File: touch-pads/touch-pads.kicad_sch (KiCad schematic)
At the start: 47 parts, among them J1 Conn_01x06_Pin, J2 Conn_01x06_Socket, J3 Conn_01x06_Pin, K1 Conn_01x01, K10 Conn_01x01, K11 Conn_01x01, K12 Conn_01x01, K13 Conn_01x01, K14 Conn_01x01, K15 Conn_01x01, K16 Conn_01x01, K17 Conn_01x01, K18 Conn_01x01, K19 Conn_01x01, K2 Conn_01x01, K20 Conn_01x01, K21 Conn_01x01, K22 Conn_01x01, K23 Conn_01x01, K24 Conn_01x01, K25 Conn_01x01, K26 Conn_01x01, K27 Conn_01x01, K28 Conn_01x01, K29 Conn_01x01, K3 Conn_01x01, K30 Conn_01x01, K31 Conn_01x01, K32 Conn_01x01, K4 Conn_01x01, K5 Conn_01x01, K6 Conn_01x01, K7 Conn_01x01, K8 Conn_01x01, K9 Conn_01x01, U10 CAP1188-1-CP-TR, U11 CAP1188-1-CP-TR, U8 CAP1188-1-CP-TR, U9 CAP1188-1-CP-TR

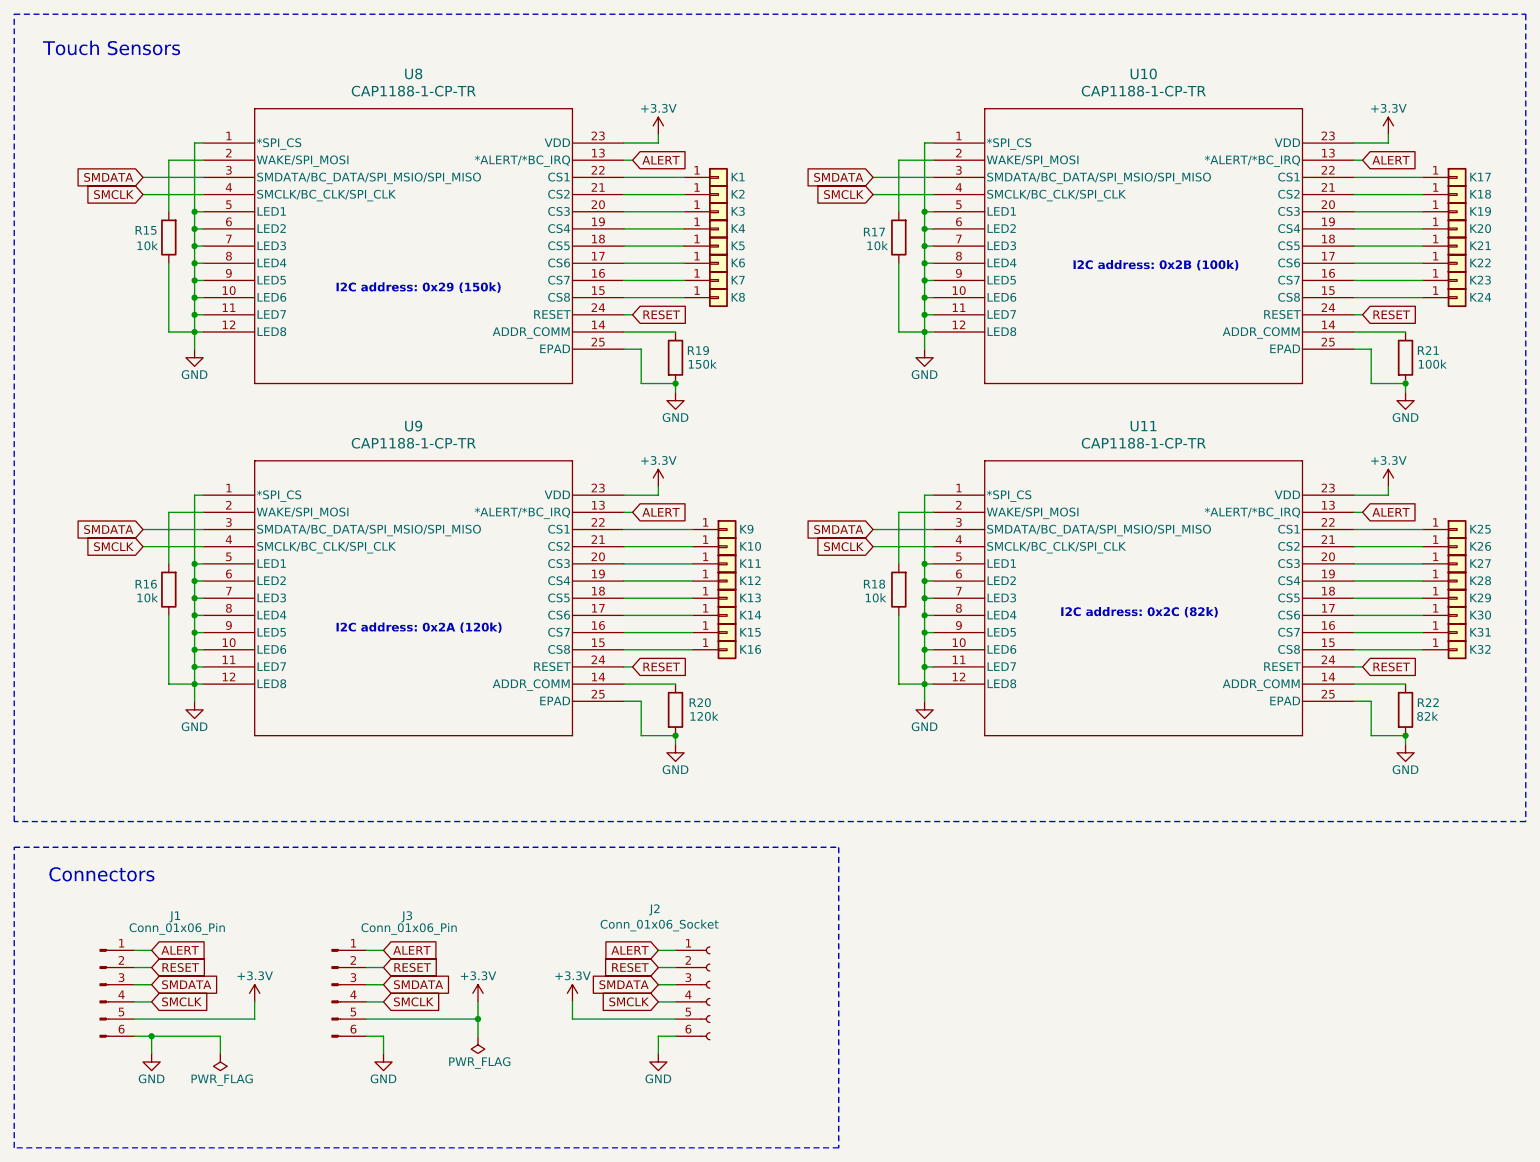
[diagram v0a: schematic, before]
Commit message: small board
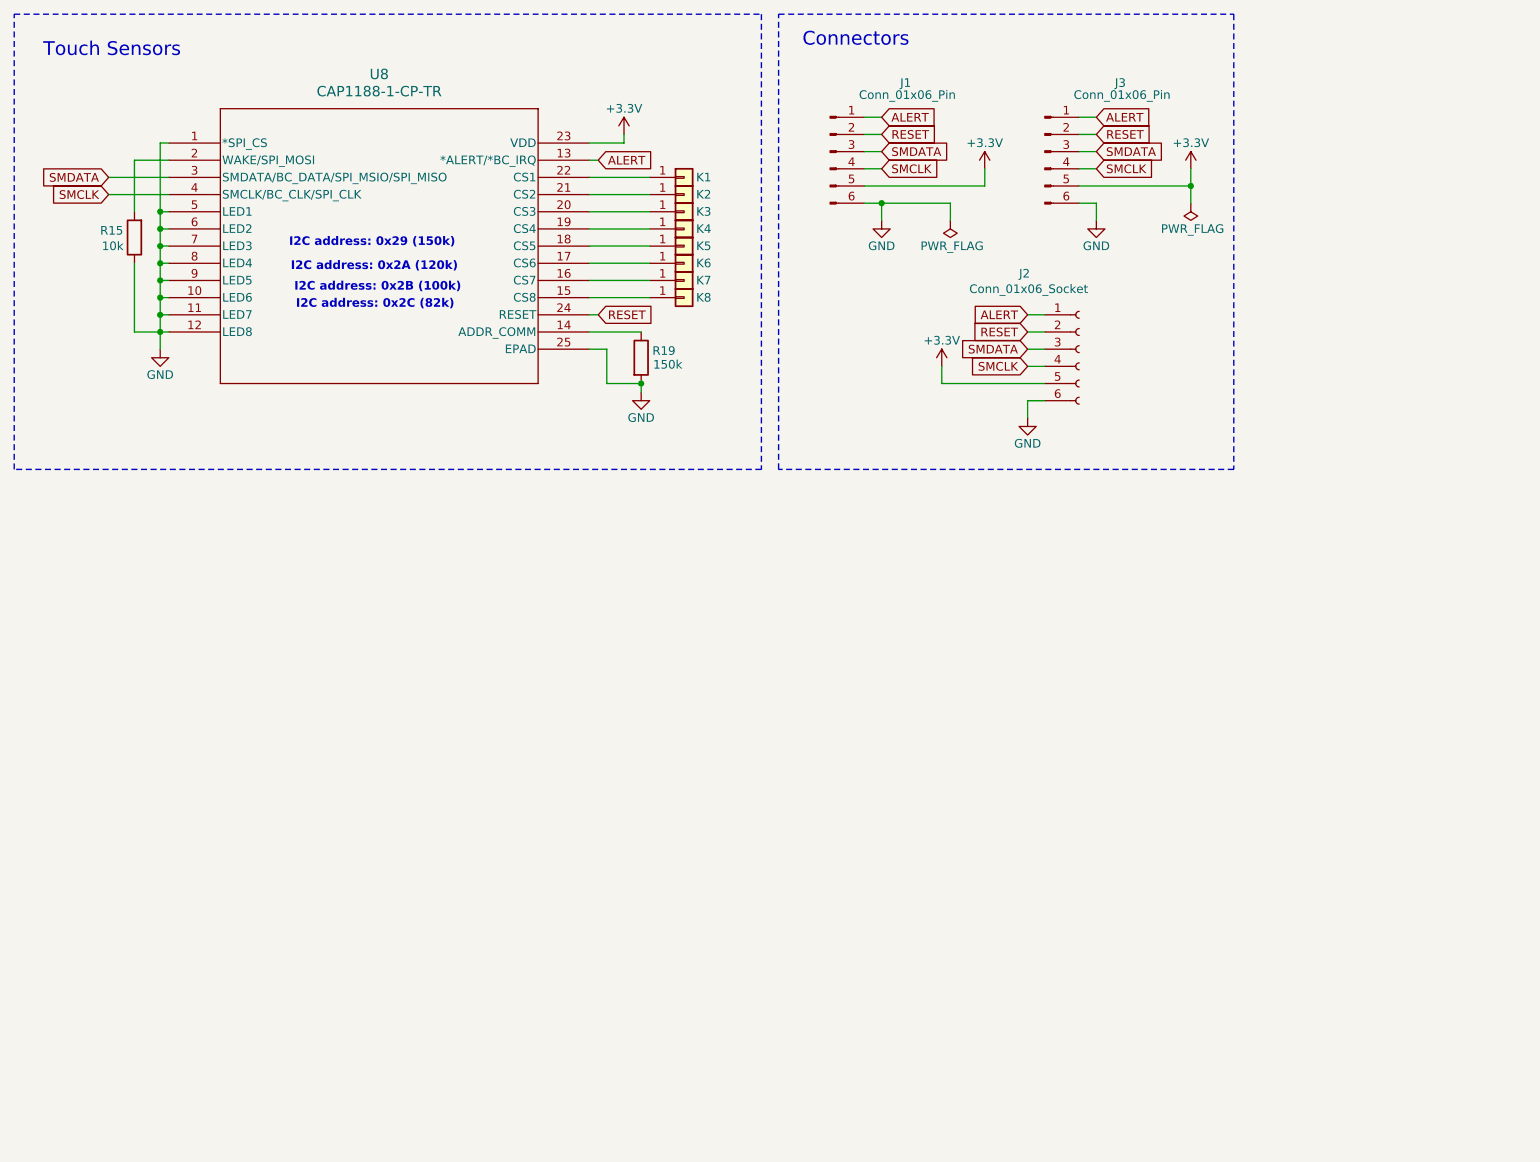
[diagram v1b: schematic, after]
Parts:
- removed K10, K11, K12, K13, K14, K15, K16, K17, K18, K19, K20, K21, K22, K23, K24, K25, K26, K27, K28, K29, K30, K31, K32, K9: Conn_01x01, TouchKey:TouchKey_Standard, symbol Connector_Generic:Conn_01x01
- removed R16, R17, R18: 10k, Resistor_SMD:R_0805_2012Metric_Pad1.20x1.40mm_HandSolder, symbol Device:R
- removed R20: 120k, Resistor_SMD:R_0805_2012Metric_Pad1.20x1.40mm_HandSolder, symbol Device:R
- removed R21: 100k, Resistor_SMD:R_0805_2012Metric_Pad1.20x1.40mm_HandSolder, symbol Device:R
- removed R22: 82k, Resistor_SMD:R_0805_2012Metric_Pad1.20x1.40mm_HandSolder, symbol Device:R
- removed U10, U11, U9: CAP1188-1-CP-TR, CAP1188_1_CP_TR:QFN24_4X4MC_MCH, symbol CAP1188_1_CP_TR:CAP1188-1-CP-TR
- J1, J3: footprint (none) -> Connector_PinHeader_2.54mm:PinHeader_1x06_P2.54mm_Horizontal
- J2: footprint (none) -> Connector_PinSocket_2.54mm:PinSocket_1x06_P2.54mm_Horizontal
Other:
- moved on the sheet: J1, J2, J3, K1, K2, K3, K4, K5, K6, K7, K8, R15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

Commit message: large board
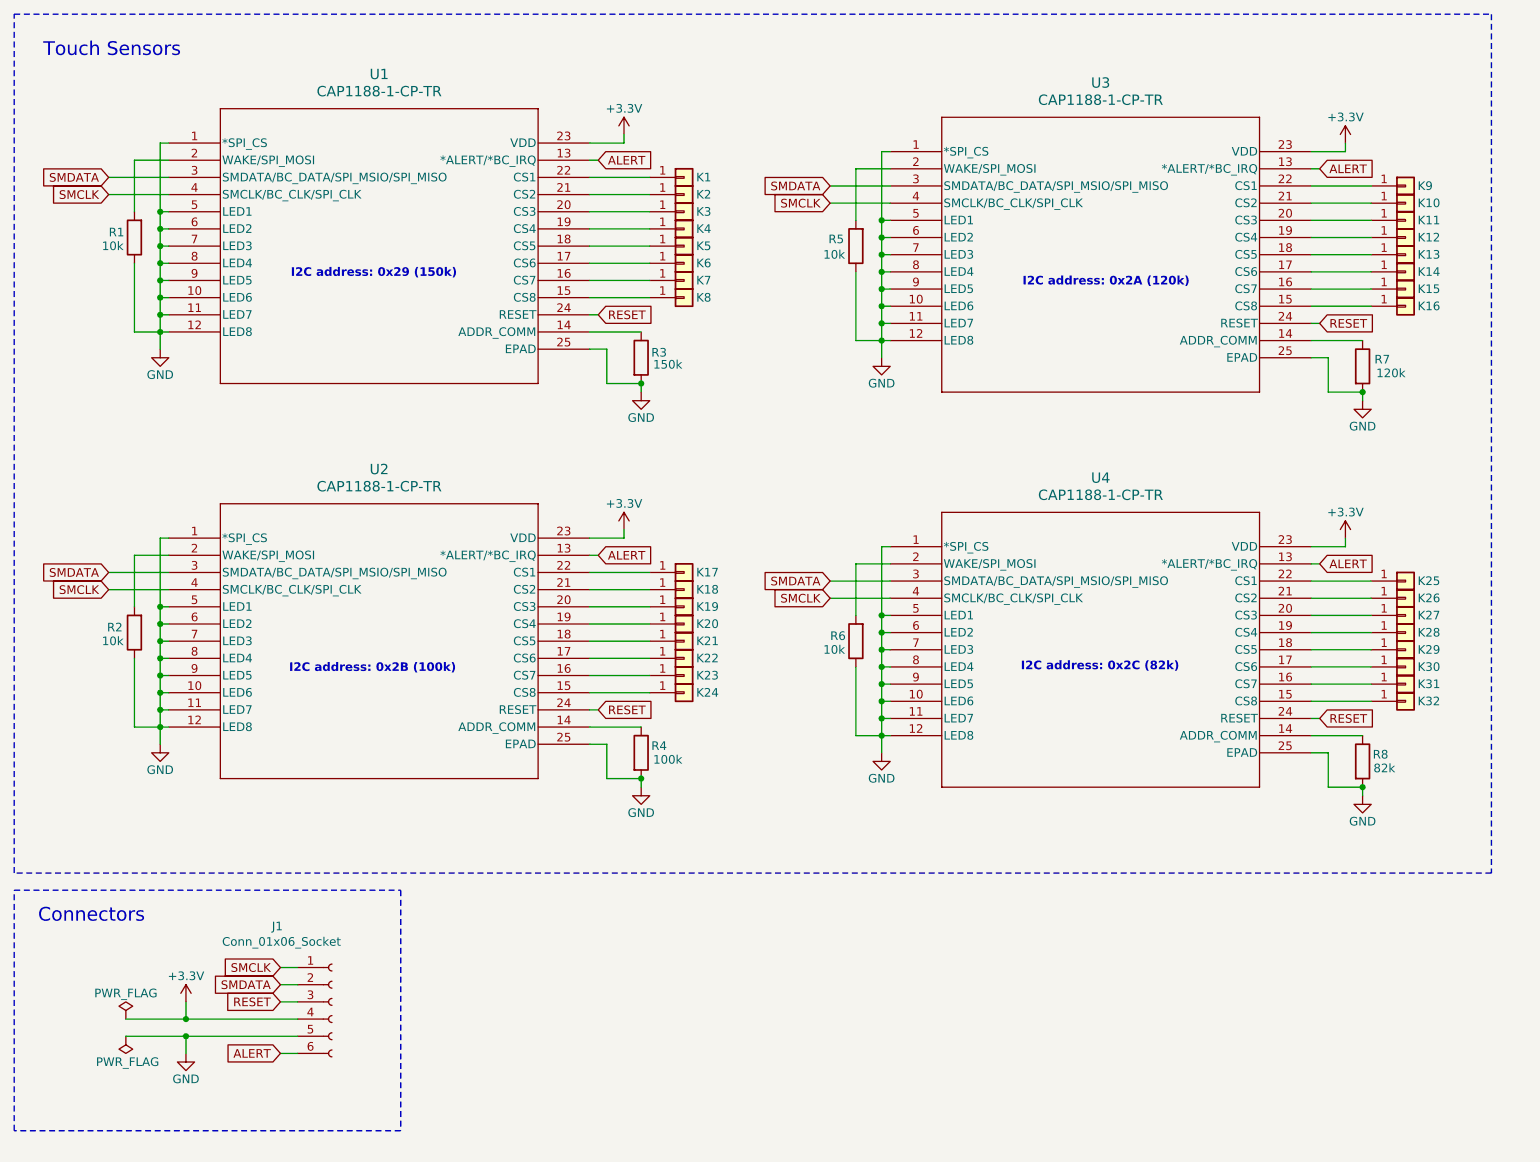
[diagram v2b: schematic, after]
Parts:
- removed J1, J3: Conn_01x06_Pin, Connector_PinHeader_2.54mm:PinHeader_1x06_P2.54mm_Horizontal, symbol Connector:Conn_01x06_Pin
- added K10, K11, K12, K13, K14, K15, K16, K17, K18, K19, K20, K21, K22, K23, K24, K25, K26, K27, K28, K29, K30, K31, K32, K9: Conn_01x01, TouchKey:TouchKey_Standard, symbol Connector_Generic:Conn_01x01
- added R2, R5, R6: 10k, Resistor_SMD:R_0805_2012Metric_Pad1.20x1.40mm_HandSolder, symbol Device:R
- added R4: 100k, Resistor_SMD:R_0805_2012Metric_Pad1.20x1.40mm_HandSolder, symbol Device:R
- added R7: 120k, Resistor_SMD:R_0805_2012Metric_Pad1.20x1.40mm_HandSolder, symbol Device:R
- added R8: 82k, Resistor_SMD:R_0805_2012Metric_Pad1.20x1.40mm_HandSolder, symbol Device:R
- added U2, U3, U4: CAP1188-1-CP-TR, CAP1188_1_CP_TR:QFN24_4X4MC_MCH, symbol CAP1188_1_CP_TR:CAP1188-1-CP-TR
- J1: renamed from J2; footprint Connector_PinSocket_2.54mm:PinSocket_1x06_P2.54mm_Horizontal -> Connector_JST:JST_XH_B6B-XH-A_1x06_P2.50mm_Vertical
- renumbered R15 to R1, R19 to R3, U8 to U1
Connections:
- net +3.3V: now also J1.4 (Pin_4), U2.23 (VDD), U3.23 (VDD), U4.23 (VDD); no longer J1.5 (Pin_5)
- net ALERT: now also J1.6 (Pin_6), U2.13 (*ALERT/*BC_IRQ), U3.13 (*ALERT/*BC_IRQ), U4.13 (*ALERT/*BC_IRQ); no longer J1.1 (Pin_1)
- net GND: now also J1.5 (Pin_5), R2.1, R4.2, R5.1, R6.1, R7.2, R8.2, U2.1 (*SPI_CS), U2.10 (LED6), U2.11 (LED7), U2.12 (LED8), U2.25 (EPAD), U2.5 (LED1), U2.6 (LED2), U2.7 (LED3), U2.8 (LED4), U2.9 (LED5), U3.1 (*SPI_CS), U3.10 (LED6), U3.11 (LED7), U3.12 (LED8), U3.25 (EPAD), U3.5 (LED1), U3.6 (LED2), U3.7 (LED3), U3.8 (LED4), U3.9 (LED5), U4.1 (*SPI_CS), U4.10 (LED6), U4.11 (LED7), U4.12 (LED8), U4.25 (EPAD), U4.5 (LED1), U4.6 (LED2), U4.7 (LED3), U4.8 (LED4), U4.9 (LED5); no longer J1.6 (Pin_6)
- net RESET: now also J1.3 (Pin_3), U2.24 (RESET), U3.24 (RESET), U4.24 (RESET); no longer J1.2 (Pin_2)
- net SMCLK: now also J1.1 (Pin_1), U2.4 (SMCLK/BC_CLK/SPI_CLK), U3.4 (SMCLK/BC_CLK/SPI_CLK), U4.4 (SMCLK/BC_CLK/SPI_CLK); no longer J1.4 (Pin_4)
- net SMDATA: now also J1.2 (Pin_2), U2.3 (SMDATA/BC_DATA/SPI_MSIO/SPI_MISO), U3.3 (SMDATA/BC_DATA/SPI_MSIO/SPI_MISO), U4.3 (SMDATA/BC_DATA/SPI_MSIO/SPI_MISO); no longer J1.3 (Pin_3)
- new net: K19.1 (Pin_1), U2.20 (CS3)
- new net: K12.1 (Pin_1), U3.19 (CS4)
- new net: R6.2, U4.2 (WAKE/SPI_MOSI)
- new net: K13.1 (Pin_1), U3.18 (CS5)
- new net: K29.1 (Pin_1), U4.18 (CS5)
- new net: K25.1 (Pin_1), U4.22 (CS1)
- new net: K14.1 (Pin_1), U3.17 (CS6)
- new net: R7.1, U3.14 (ADDR_COMM)
- new net: K16.1 (Pin_1), U3.15 (CS8)
- new net: K15.1 (Pin_1), U3.16 (CS7)
- new net: R5.2, U3.2 (WAKE/SPI_MOSI)
- new net: K11.1 (Pin_1), U3.20 (CS3)
- new net: K10.1 (Pin_1), U3.21 (CS2)
- new net: K9.1 (Pin_1), U3.22 (CS1)
- new net: K21.1 (Pin_1), U2.18 (CS5)
- new net: R2.2, U2.2 (WAKE/SPI_MOSI)
- new net: K31.1 (Pin_1), U4.16 (CS7)
- new net: K23.1 (Pin_1), U2.16 (CS7)
- new net: K32.1 (Pin_1), U4.15 (CS8)
- new net: R8.1, U4.14 (ADDR_COMM)
- new net: K30.1 (Pin_1), U4.17 (CS6)
- new net: K28.1 (Pin_1), U4.19 (CS4)
- new net: K27.1 (Pin_1), U4.20 (CS3)
- new net: K26.1 (Pin_1), U4.21 (CS2)
- new net: K17.1 (Pin_1), U2.22 (CS1)
- new net: K22.1 (Pin_1), U2.17 (CS6)
- new net: R4.1, U2.14 (ADDR_COMM)
- new net: K24.1 (Pin_1), U2.15 (CS8)
- new net: K20.1 (Pin_1), U2.19 (CS4)
- new net: K18.1 (Pin_1), U2.21 (CS2)
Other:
- moved on the sheet: J1
